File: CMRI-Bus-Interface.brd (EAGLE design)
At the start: 50 x 50 mm, 15 parts, among them U3 NE555P, U4 MAX3465CPD

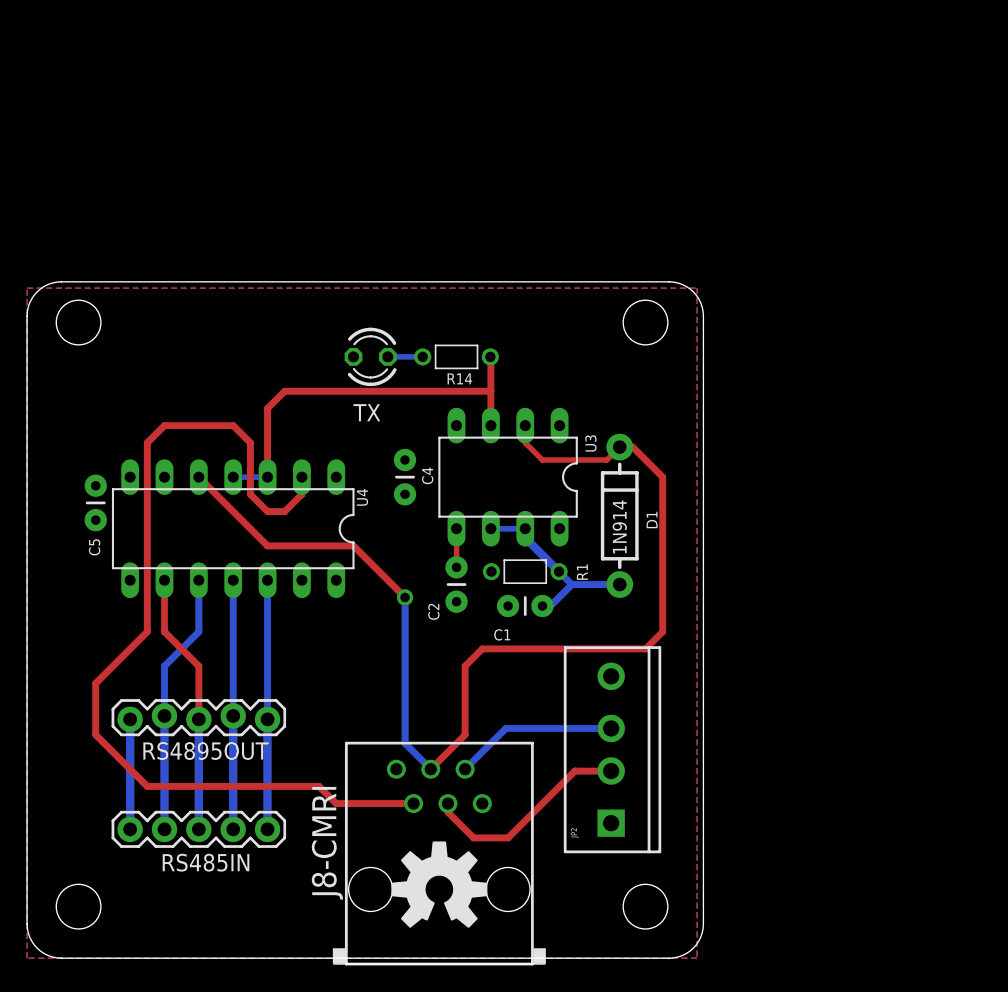
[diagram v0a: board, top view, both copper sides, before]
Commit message: 2.0
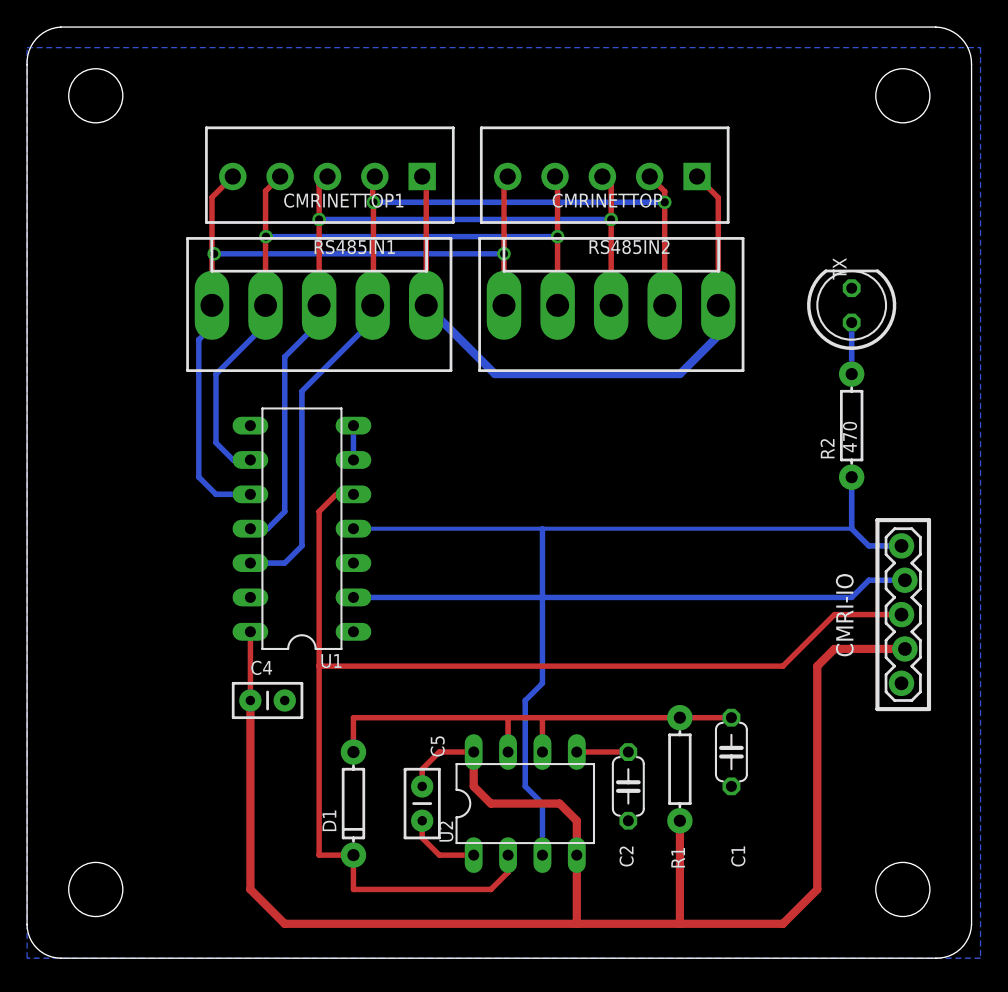
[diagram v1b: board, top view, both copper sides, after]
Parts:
- removed J8-CMRI: (no value), SPCoast:RJ11-NO_SHIELD
- removed JP2: (no value), SparkFun-Connectors:SCREWTERMINAL-3.5MM-4_LOCK
- removed R14: 1k0, SPCoast:1/6W-RES
- removed RS485IN: (no value), SparkFun:1X05
- removed RS4895OUT: (no value), SparkFun:1X05_LOCK
- removed U$1: OSHW-LOGOL, SparkFun:OSHW-LOGO-L
- removed U3: NE555P, SparkFun:DIL-08
- removed U4: MAX3465CPD, maxim:DIL14
- added BOARD1: BOARD69X70, SPCoast:BOARD-DINRAIL-2.7IN-7CM
- added CMRI-IO: (no value), SPCoast:CON-CMRI-IO
- added CMRINETTOP, CMRINETTOP1: (no value), SPCoast:CMRINET-3.5MM
- added R2: 470, SPCoast:AXIAL-0.3-RES
- added RS485IN1: CMRInet Hdr Rt, SPCoast:KK-156-5
- added RS485IN2: CMRInet Hdr Top, SPCoast:KK-156-5
- added U$3: (no value), SPCoast:MRCS-LOGO
- added U1: MAX3465CPD, SPCoast:DIL14
- added U2: (no value), SPCoast:DIL-08
- C1, C2: device SPCoast:CAP-PTH-SMALL -> SPCoast:C050-024X044
- C4, C5: value .1uF -> .01uF; device SPCoast:CAP-PTH-SMALL -> SPCoast:C-PTH-0.100
- D1: value 1N914 -> 1N4148; device MCP:DIODE-1N4001 -> SPCoast:DIODE-1N4148
- R1: device SPCoast:1/6W-RES -> SPCoast:AXIAL-0.3-RES
- TX: value LEDLED3MM -> (none); device SPCoast:LED3MM -> SPCoast:LED5MM
- moved TX 35.8 mm to (61.0, 48.3), turned to 90 degrees
- moved C5 32.0 mm to (29.2, 11.4), turned to 270 degrees
- moved D1 29.0 mm to (24.1, 11.4)
- moved C2 20.6 mm to (44.5, 12.7)
- moved C4 20.5 mm to (17.8, 19.1), turned to 0 degrees
- moved R1 18.5 mm to (48.3, 14.0), turned to 270 degrees
- moved C1 17.7 mm to (52.1, 15.2), turned to 270 degrees
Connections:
- removed net IN+: RS485IN.1, RS4895OUT.1, U4.12
- removed net IN-: RS485IN.2, RS4895OUT.2, U4.11
- removed net N$1: C1.1, D1.A, R1.1, U3.6, U3.7
- removed net N$2: J8-CMRI.4, JP2.2
- removed net N$3: J8-CMRI.5, JP2.3
- removed net OUT+: RS485IN.3, RS4895OUT.3, U4.9
- removed net OUT-: RS485IN.4, RS4895OUT.4, U4.10
- removed net RXD: J8-CMRI.2, U4.2
- removed net TXD: D1.C, J8-CMRI.3, U3.2, U4.5
- new net N$36: CMRINETTOP.4, CMRINETTOP1.4, RS485IN1.4, RS485IN2.4, U1.12
- new net N$52: C1.1, D1.A, R1.P$1, U2.6, U2.7
- new net N$56: CMRINETTOP.3, CMRINETTOP1.3, RS485IN1.3, RS485IN2.3, U1.11
- new net N$59: CMRINETTOP.2, CMRINETTOP1.2, RS485IN1.2, RS485IN2.2, U1.9
- new net N$60: CMRINETTOP.1, CMRINETTOP1.1, RS485IN1.1, RS485IN2.1, U1.10
- new net RX: CMRI-IO.4, U1.2
- new net TX: CMRI-IO.3, D1.C, U1.5, U2.2
- net GND: now also CMRI-IO.1, U1.3, U1.6, U1.7, U2.1; no longer J8-CMRI.6, JP2.4, U3.1, U4.6, U4.7
- net N$29: now also R2.P$2; no longer R14.2
- net N$38: now also U2.5; no longer U3.5
- net SHIELD: now also CMRINETTOP.5, CMRINETTOP1.5, RS485IN1.5, RS485IN2.5; no longer RS485IN.5, RS4895OUT.5
- net TXEN: now also CMRI-IO.5, R2.P$1, U1.4, U2.3; no longer R14.1, U3.3, U4.3, U4.4
- net VCC: now also CMRI-IO.2, R1.P$2, U1.14, U2.4, U2.8; no longer J8-CMRI.1, JP2.1, R1.2, U3.4, U3.8, U4.14
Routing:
- net VCC: track 0.00 -> 118.6 mm
- net TX: track 0.00 -> 90.1 mm
- net TXD: track 81.4 -> 0.00 mm, vias 1 -> 0
- net RXD: track 67.4 -> 0.00 mm
- net N$36: track 0.00 -> 65.4 mm, vias 0 -> 2
- net N$56: track 0.00 -> 60.5 mm, vias 0 -> 2
- net N$60: track 0.00 -> 58.9 mm, vias 0 -> 2
- net N$59: track 0.00 -> 56.0 mm, vias 0 -> 2
- net RX: track 0.00 -> 41.3 mm
- net TXEN: track 29.8 -> 70.0 mm
- net SHIELD: track 8.13 -> 46.9 mm
- net N$52: track 0.00 -> 35.6 mm
- net OUT-: track 19.5 -> 0.00 mm
- net OUT+: track 19.5 -> 0.00 mm
- net IN-: track 18.4 -> 0.00 mm
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- removed copper zone on layer 1, net VCC
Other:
- board size 50 x 50 mm -> 69.8 x 68.8 mm
- board text added: "115200 1000 0.1 uF"
- board text added: "19200 12000 0.1 uF"
- board text added: "2019-07"
- board text added: "28800 3300 0.1 uF"
- board text added: "38400 3000 0.1 uF"
- board text added: "57600 2000 0.1 uF"
- board text added: "9600 12000 0.1 uF"
- board text added: "AutoRTS - Optional"
- board text added: "AutoRTS Values"
- board text added: "BPS R1 C1"
- board text added: "CMRI Interface"
- board text added: "MRCS Design"
- board text added: "v2.0p"
- board text removed: "2014.07"
- board text removed: "4-wire"
- board text removed: "5V"
- board text removed: "5v"
- board text removed: "C/MRI Interface"
- board text removed: "D0 RX"
- board text removed: "D1 TX"
- board text removed: "D2 nc"
- board text removed: "D3 nc"
- board text removed: "GND"
- board text removed: "Go Bears!"
- board text removed: "IN+"
- board text removed: "IN-"
- board text removed: "IO-CMRI"
- board text removed: "John Plocher"
- board text removed: "Made in the PCR, Coast Division, NMRA"
- board text removed: "Model Railroading is fun!"
- board text removed: "Out+"
- board text removed: "Out-"
- board text removed: "RS-485"
- board text removed: "RS485 adapter"
- board text removed: "Shield"
- board text removed: "gnd"
- board text removed: "v1.0"
- board text removed: "www. SP Coast .com"
